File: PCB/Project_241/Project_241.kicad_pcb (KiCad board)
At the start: 2 copper layers, 55 x 60 mm, 40 parts, among them J2 Wind_Hall, J4 SPI CONNECTOR, J5 Rain_Hall, J6 BATT_CONN, SW1 RESET, U1 STM32F103C8T6, U3 LM393, U4 RA02, U5 HDC1080, U7 RT9013

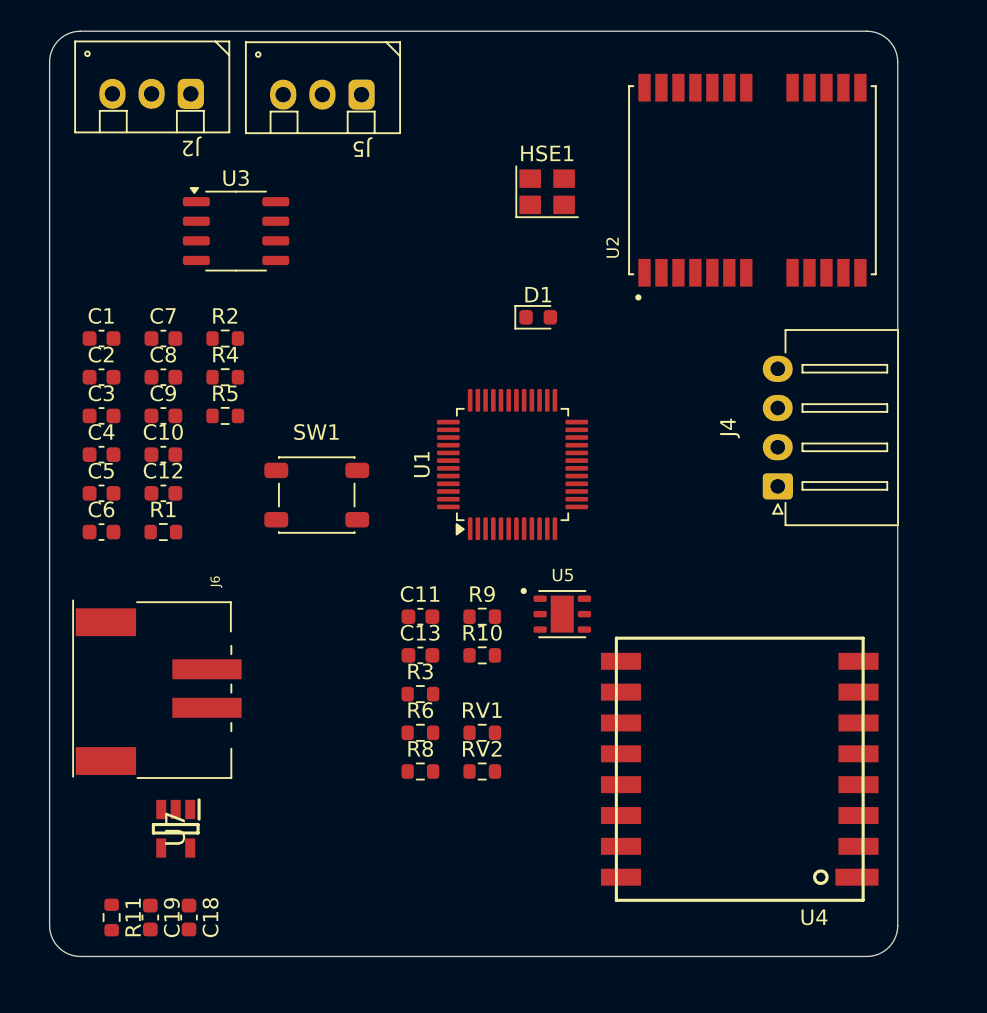
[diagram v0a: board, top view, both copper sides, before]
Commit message: update gerber
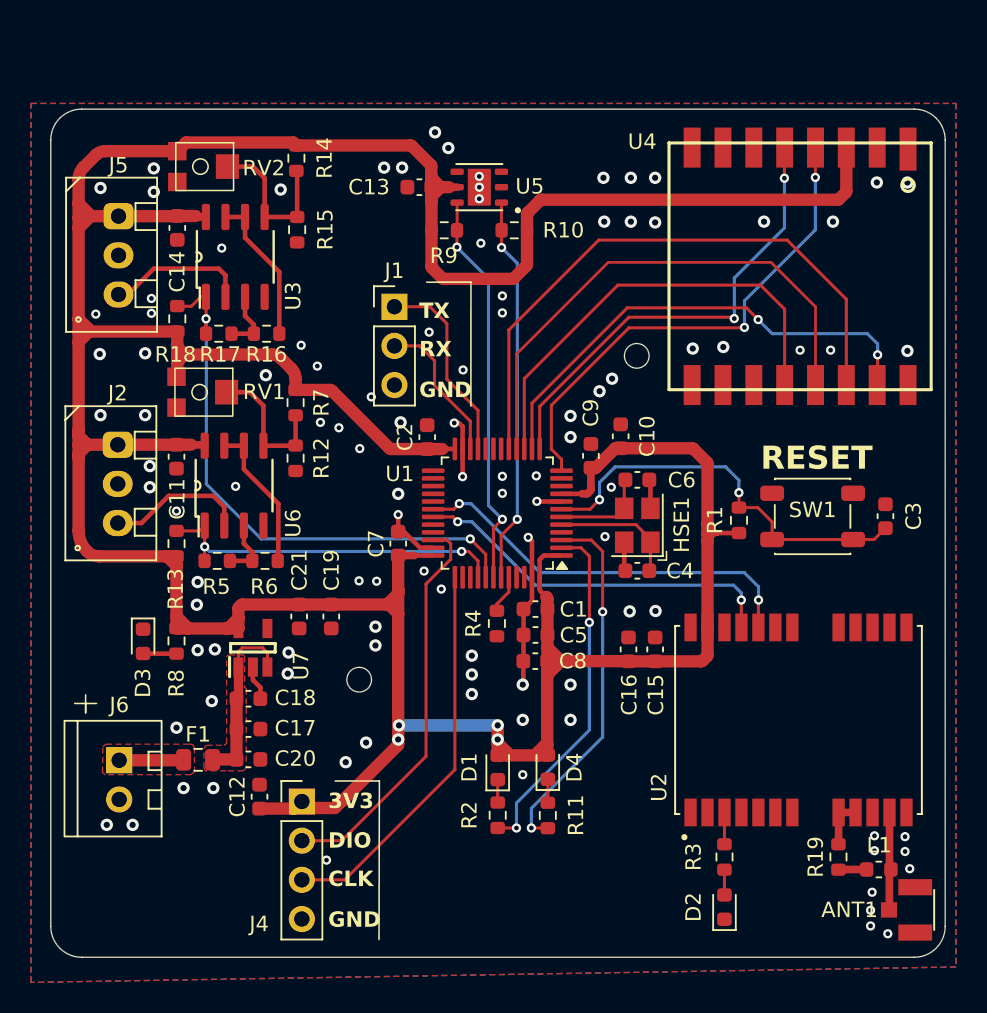
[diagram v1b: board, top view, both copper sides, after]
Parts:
- added ANT1: IPEX_SMA, project241_footprint:ANT_SMA_3PIN, F.Cu at (187.4, 128.3)
- added C14: 100nF, Capacitor_SMD:C_0603_1608Metric, F.Cu at (139.5, 84.1)
- added C15: 4.7uF, Capacitor_SMD:C_0603_1608Metric, F.Cu at (170.5, 111.4)
- added C16: 100nF, Capacitor_SMD:C_0603_1608Metric, F.Cu at (168.8, 111.4)
- added C17: 10uF, Capacitor_SMD:C_0603_1608Metric, F.Cu at (144.1, 116.6)
- added C20: 100nF, Capacitor_SMD:C_0603_1608Metric, F.Cu at (144.1, 118.5)
- added C21: 100nF, Capacitor_SMD:C_0603_1608Metric, F.Cu at (147.4, 109.3)
- added D2: RED_LED, LED_SMD:LED_0603_1608Metric, F.Cu at (175.0, 128.1)
- added D3: PWR_LED, LED_SMD:LED_0603_1608Metric, F.Cu at (137.3, 110.9)
- added D4: GREEN_LED, LED_SMD:LED_0603_1608Metric, F.Cu at (163.5, 119.0)
- added F1: 1A, Fuse:Fuse_0805_2012Metric, F.Cu at (140.8, 118.6)
- added J1: UART_CONNECTOR, Connector_PinHeader_2.54mm:PinHeader_1x03_P2.54mm_Vertical, F.Cu at (153.6, 89.2)
- added L1: 27nH, Inductor_SMD:L_0603_1608Metric, F.Cu at (185.0, 125.7)
- added R12: DNP, Resistor_SMD:R_0603_1608Metric, F.Cu at (147.2, 99.0)
- added R13: 2k2, Resistor_SMD:R_0603_1608Metric, F.Cu at (139.4, 104.5)
- added R14: DNP, Resistor_SMD:R_0603_1608Metric, F.Cu at (147.2, 79.6)
- added R15: DNP, Resistor_SMD:R_0603_1608Metric, F.Cu at (147.3, 84.2)
- added R16: 1k, Resistor_SMD:R_0603_1608Metric, F.Cu at (145.3, 90.9)
- added R17: 15k, Resistor_SMD:R_0603_1608Metric, F.Cu at (142.2, 90.9)
- added R18: 2k2, Resistor_SMD:R_0603_1608Metric, F.Cu at (139.5, 90.0)
- added R19: 22R, Resistor_SMD:R_0603_1608Metric, F.Cu at (182.4, 124.9)
- added R7: DNP, Resistor_SMD:R_0603_1608Metric, F.Cu at (147.2, 95.4)
- added U6: LM358, IVSFootprint:SOIC-8, F.Cu at (143.2, 100.8)
- J4: footprint IVSFootprint:XH_4P_2.54mm_Horizontal -> Connector_PinHeader_2.54mm:PinHeader_1x04_P2.54mm_Vertical
- J6: footprint IVSFootprint:XH_2P_2.54mm_Horizontal_SMD -> IVSFootprint:XH 2.54 2Pin Female
- R11: value 10k -> 56R
- R3, R8: value 1k -> 100R
- R5: value 1k -> 15k
- RV1, RV2: footprint Resistor_SMD:R_0603_1608Metric -> project241_footprint:Poten_3PIN_SMD
- U2: value ~ -> NEO 6M
- U3: value LM393 -> LM358; footprint Package_SO:SO-8_3.9x4.9mm_P1.27mm -> IVSFootprint:SOIC-8
- moved C3 51.2 mm to (185.4, 102.8), turned to 90 degrees
- moved RV2 44.8 mm to (139.5, 79.1), turned to -90 degrees
- moved J4 39.3 mm to (147.6, 121.3), turned to 0 degrees
- moved R1 37.3 mm to (175.9, 103.0), turned to -90 degrees
- moved R2 35.6 mm to (160.3, 122.2), turned to 90 degrees
- moved C4 35.6 mm to (169.3, 106.3), turned to 180 degrees
- moved U2 35.1 mm to (179.8, 116.0)
- moved C6 34.9 mm to (169.3, 100.4)
- moved C1 33.2 mm to (162.7, 108.8), turned to 180 degrees
- moved U4 32.8 mm to (179.9, 86.6), turned to -90 degrees
- moved SW1 32.2 mm to (180.7, 102.8)
- moved RV1 30.4 mm to (139.4, 93.7), turned to -90 degrees
- moved C13 30.4 mm to (155.2, 81.4)
- moved C8 30.3 mm to (162.7, 112.2), turned to 180 degrees
- moved C10 29.7 mm to (168.2, 97.6), turned to 90 degrees
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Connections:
- J6 pad 1: +BATT -> Net-(J6-Pin_1)
- R11 pad 1: +BATT -> /MCU/LED_PC14
- R11 pad 2: Net-(U7-EN) -> Net-(D4-K)
- R3 pad 1: /MCU/RAIN_GAUSE -> Net-(D2-A)
- R3 pad 2: Net-(U3B-+) -> Net-(U2-TIMEPULSE)
- R5 pad 2: Net-(U3A-+) -> Net-(U6A-+)
- R6 pad 1: Net-(U3A-+) -> Net-(U6A-+)
- R6 pad 2: Net-(R6-Pad2) -> Net-(U6B--)
- R8 pad 1: Net-(U3B-+) -> VDD
- R8 pad 2: Net-(R8-Pad2) -> Net-(D3-A)
- RV1 pad 2: Net-(R6-Pad2) -> Net-(U6B-+)
- RV2 pad 2: Net-(R8-Pad2) -> Net-(U3B-+)
- U1 pad 11: /LORA/DIO1 -> unconnected-(U1-PA1-Pad11)
- U1 pad 12: unconnected-(U1-PA2-Pad12) -> /LORA/LORA_RESET
- U1 pad 13: /LORA/RESET -> /LORA/DIO1
- U1 pad 21: unconnected-(U1-PB10-Pad21) -> /MCU/DEBUG_TX
- U1 pad 22: unconnected-(U1-PB11-Pad22) -> /MCU/DEBUG_RX
- U1 pad 3: unconnected-(U1-PC14-Pad3) -> /MCU/LED_PC14
- U1 pad 30: unconnected-(U1-PA9-Pad30) -> /MCU/GPS_TX
- U1 pad 31: unconnected-(U1-PA10-Pad31) -> /MCU/GPS_RX
- U2 pad 1: (no net) -> unconnected-(U2-RSVD_1-Pad1)
- U2 pad 10: Net-(U2-GND-Pad10) -> GND
- U2 pad 11: unconnected-(U2-RF_IN-Pad11) -> Net-(ANT1-FEED)
- U2 pad 12: Net-(U2-GND-Pad10) -> GND
- U2 pad 13: Net-(U2-GND-Pad10) -> GND
- U2 pad 20: unconnected-(U2-TXD1-Pad20) -> /MCU/GPS_TX
- U2 pad 21: unconnected-(U2-RXD1-Pad21) -> /MCU/GPS_RX
- U2 pad 23: unconnected-(U2-VCC-Pad23) -> VDD
- U2 pad 24: Net-(U2-GND-Pad10) -> GND
- U2 pad 3: unconnected-(U2-TIMEPULSE-Pad3) -> Net-(U2-TIMEPULSE)
- U2 pad 8: unconnected-(U2-RSVD_8-Pad8) -> Net-(U2-RSVD_8)
- U2 pad 9: unconnected-(U2-VCC_RF-Pad9) -> Net-(U2-RSVD_8)
- U3 pad 1: /MCU/WIND_SPEED -> /MCU/RAIN_GAUSE
- U3 pad 2: Net-(J2-Pin_3) -> Net-(J5-Pin_3)
- U3 pad 4: VDD -> GND
- U3 pad 6: Net-(J5-Pin_3) -> Net-(U3B--)
- U3 pad 7: /MCU/RAIN_GAUSE -> Net-(U3B--)
- U3 pad 8: GND -> VDD
- U4 pad 4: /LORA/RESET -> /LORA/LORA_RESET
- U7 pad 3: Net-(U7-EN) -> +BATT
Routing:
- net VDD: track 0.00 -> 274.9 mm, vias 0 -> 4
- net /LORA/MOSI: track 0.00 -> 39.2 mm
- net /MCU/RAIN_GAUSE: track 0.00 -> 37.7 mm, vias 0 -> 2
- net /LORA/MISO: track 0.00 -> 34.3 mm
- net /LORA/LORA_RESET: track 0.00 -> 32.7 mm, vias 0 -> 2
- net /LORA/NSS: track 0.00 -> 31.6 mm, vias 0 -> 2
- net /LORA/DIO1: track 0.00 -> 30.2 mm, vias 0 -> 2
- net /LORA/SCK: track 0.00 -> 29.5 mm
- net /MCU/NRST: track 0.00 -> 26.8 mm, vias 0 -> 2
- net /MCU/GPS_TX: track 0.00 -> 26.1 mm, vias 0 -> 2
- net /MCU/SWDIO: track 0.00 -> 26.0 mm
- net /MCU/SCL: track 0.00 -> 25.8 mm, vias 0 -> 2
- net /MCU/SWCLK: track 0.00 -> 25.4 mm
- net GND: track 0.00 -> 25.2 mm, vias 0 -> 103
- net /MCU/SDA: track 0.00 -> 25.2 mm, vias 0 -> 2
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- added copper zone on F.Cu, net +BATT
- added copper zone on B.Cu, net GND
- added copper zone on F.Cu, net GND
- added copper zone on F.Cu, net Net-(J6-Pin_1)
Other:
- board size 55 x 60 mm -> 58 x 55 mm
- board text added: "3V3"
- board text added: "CLK"
- board text added: "DIO"
- board text added: "GND"
- board text added: "RESET"
- board text added: "RX"
- board text added: "TX"
